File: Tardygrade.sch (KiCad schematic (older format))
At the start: 25 parts, among them J1 Conn_01x03, J2 Conn_01x03, J3 Conn_01x03, J4 Conn_01x03, Q1 FET, Q2 FET, U1 MCP1642B, U2 HUZZAH32, U3 Tinypico, U4 HallSwitch, U5 HallSwitch, U6 HallSwitch, U7 HallSwitch, X1 XpansionHeader

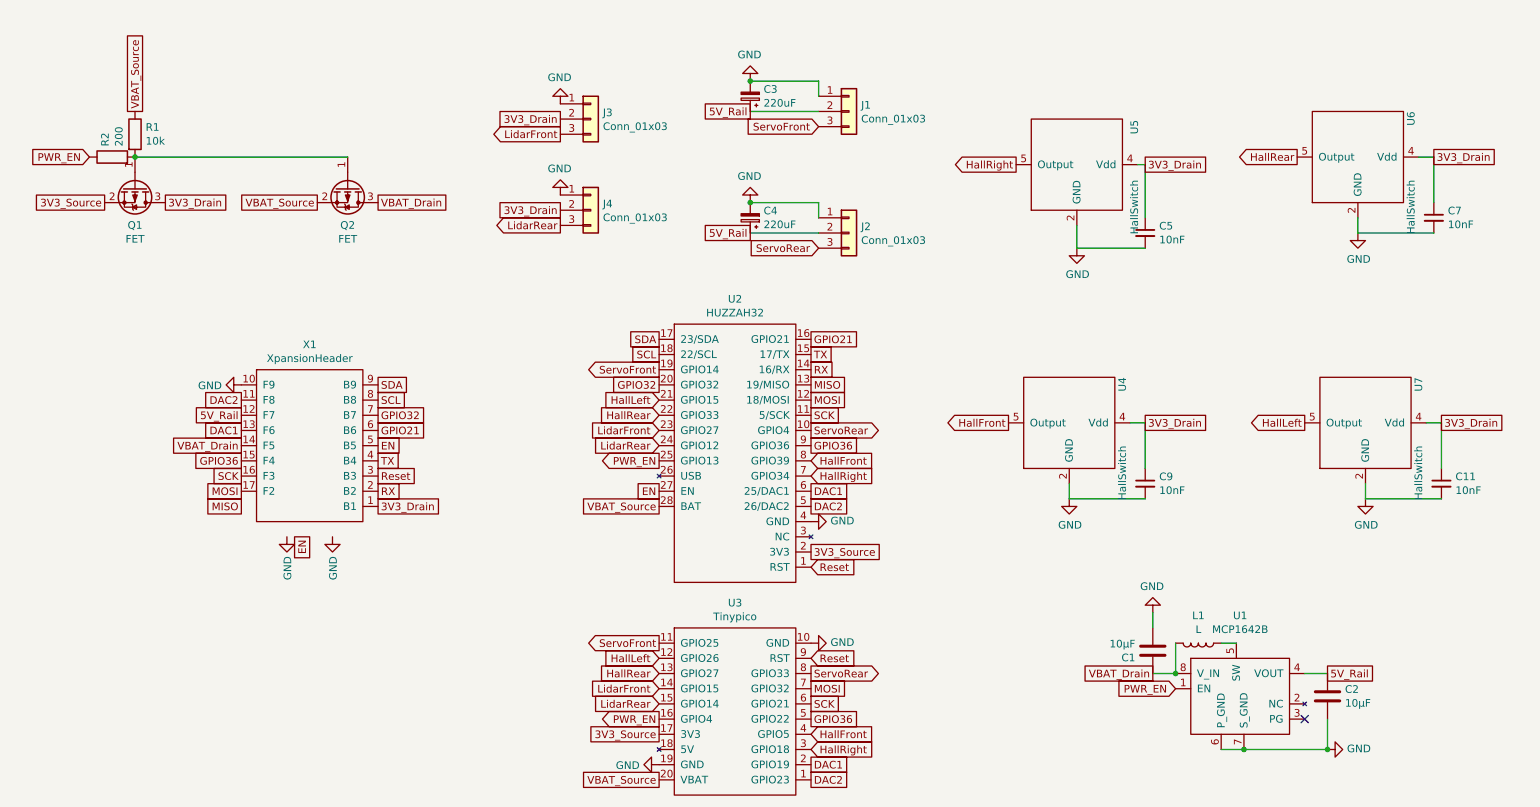
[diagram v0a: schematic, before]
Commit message: Changed some GPIOs. Minor edits.
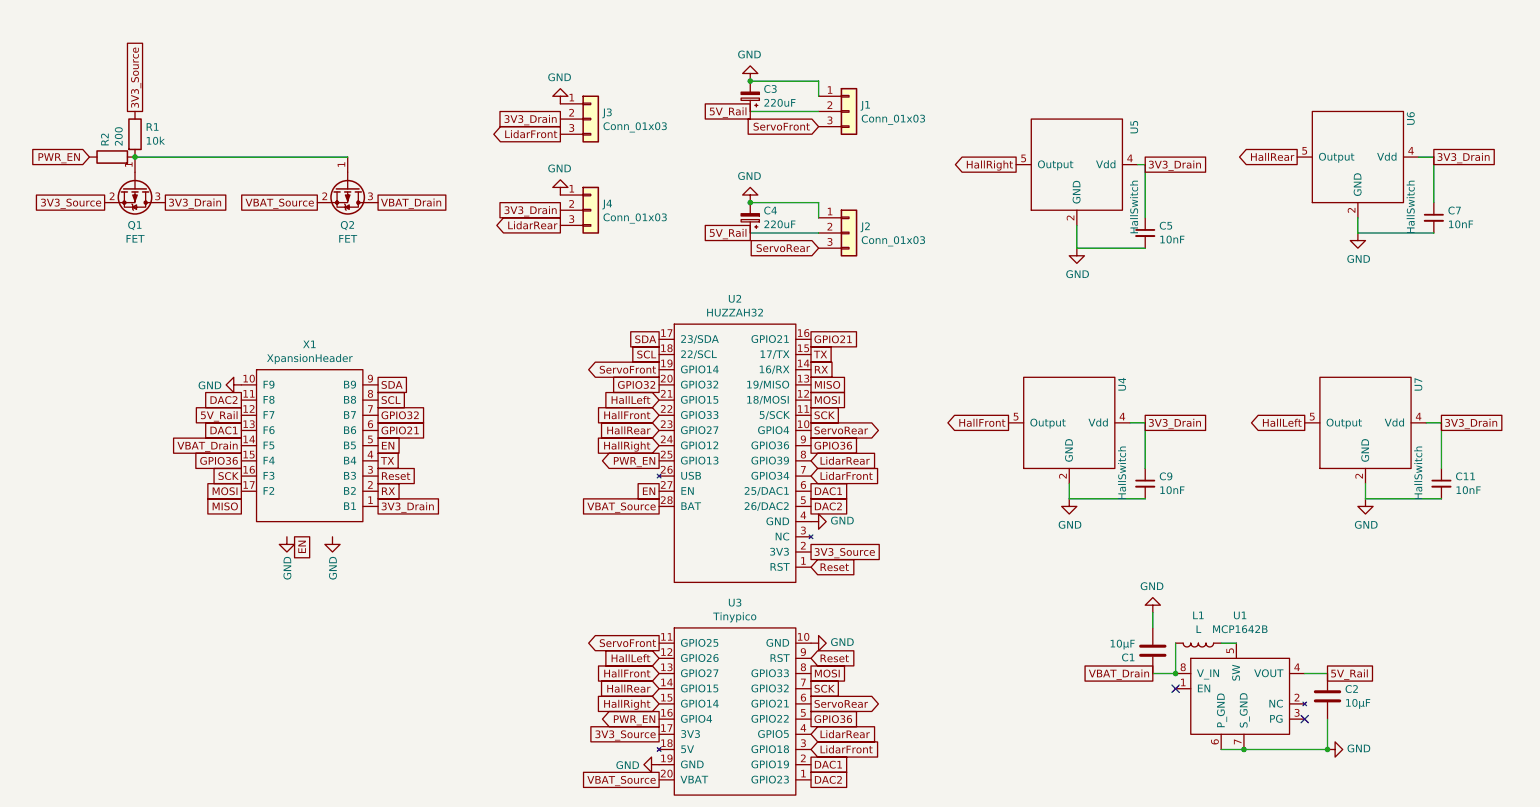
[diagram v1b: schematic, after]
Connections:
- net 3V3_Source: now also R1.1
- net HallFront: now also U2.22 (GPIO33), U3.13 (GPIO27); no longer U2.8 (GPIO39), U3.4 (GPIO5)
- net HallRear: now also U2.23 (GPIO27), U3.14 (GPIO15); no longer U2.22 (GPIO33), U3.13 (GPIO27)
- net HallRight: now also U2.24 (GPIO12), U3.15 (GPIO14); no longer U2.7 (GPIO34), U3.3 (GPIO18)
- net LidarFront: now also U2.7 (GPIO34), U3.3 (GPIO18); no longer U2.23 (GPIO27), U3.14 (GPIO15)
- net LidarRear: now also U2.8 (GPIO39), U3.4 (GPIO5); no longer U2.24 (GPIO12), U3.15 (GPIO14)
- net MOSI: now also U3.8 (GPIO33); no longer U3.7 (GPIO32)
- net PWR_EN: no longer U1.1 (EN)
- net SCK: now also U3.7 (GPIO32); no longer U3.6 (GPIO21)
- net ServoRear: now also U3.6 (GPIO21); no longer U3.8 (GPIO33)
- net VBAT_Source: no longer R1.1
- no-connect marks 1 -> 2
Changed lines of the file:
@@
 encoding utf-8
 Sheet 1 1
-Title ""
-Date ""
+Title "Tardygrade pcb v0.31"
+Date "2021-10-11"
 Rev ""
 Comp ""
@@
 Text GLabel 9750 3250 0    50   Output ~ 0
 HallLeft
-Text GLabel 5500 3200 0    50   Input ~ 0
+Text GLabel 5500 3300 0    50   Input ~ 0
 HallRear
 Text GLabel 9700 1500 0    50   Output ~ 0
 HallRear
-Text GLabel 6500 5300 2    50   Input ~ 0
+Text GLabel 5500 4900 0    50   Input ~ 0
 HallFront
-Text GLabel 6500 3500 2    50   Input ~ 0
+Text GLabel 5500 3200 0    50   Input ~ 0
 HallFront
 Text GLabel 7800 3250 0    50   Output ~ 0
 HallFront
-Text GLabel 6500 5400 2    50   Input ~ 0
+Text GLabel 5500 5100 0    50   Input ~ 0
 HallRight
-Text GLabel 6500 3600 2    50   Input ~ 0
+Text GLabel 5500 3400 0    50   Input ~ 0
 HallRight
 Text GLabel 7850 1550 0    50   Output ~ 0
@@
 Text GLabel 4850 1350 0    50   Output ~ 0
 LidarFront
-Text GLabel 5500 3300 0    50   Input ~ 0
+Text GLabel 6500 3600 2    50   Input ~ 0
 LidarFront
 $Comp
@@
 Text GLabel 1750 1500 0    50   Input ~ 0
 PWR_EN
-Text GLabel 8900 5000 0    50   Input ~ 0
-PWR_EN
 $Comp
 L power:GND #PWR0105
@@
 	0    -1   -1   0
 $EndComp
+Text GLabel 6500 5400 2    50   Input ~ 0
+LidarFront
+Text GLabel 6500 5100 2    50   Output ~ 0
+ServoRear
 Text GLabel 5500 5000 0    50   Input ~ 0
-LidarFront
-Text GLabel 6500 4900 2    50   Output ~ 0
-ServoRear
-Text GLabel 5500 4900 0    50   Input ~ 0
 HallRear
 $Comp
@@
 Text GLabel 4850 1950 0    50   Output ~ 0
 LidarRear
-Text GLabel 5500 5100 0    50   Input ~ 0
+Text GLabel 6500 5300 2    50   Input ~ 0
 LidarRear
-Text GLabel 5500 3400 0    50   Input ~ 0
+Text GLabel 6500 3500 2    50   Input ~ 0
 LidarRear
 Text GLabel 6500 3300 2    50   Output ~ 0
@@
 Text GLabel 1850 1800 0    50   UnSpc ~ 0
 3V3_Source
-Text GLabel 3250 1800 0    50   UnSpc ~ 0
-VBAT_Source
 Text GLabel 8750 4900 0    50   UnSpc ~ 0
 VBAT_Drain
@@
 Text GLabel 6500 4800 2    50   Input ~ 0
 Reset
-Text GLabel 2050 1200 1    50   UnSpc ~ 0
-VBAT_Source
 Text GLabel 3650 3400 2    50   UnSpc ~ 0
 EN
@@
 	1    0    0    -1
 $EndComp
+Text GLabel 6500 4900 2    50   UnSpc ~ 0
+MOSI
 Text GLabel 6500 5000 2    50   UnSpc ~ 0
-MOSI
-Text GLabel 6500 5100 2    50   UnSpc ~ 0
 SCK
 Text GLabel 6500 5200 2    50   UnSpc ~ 0
@@
 	6550 1800 6550 1900
 Connection ~ 6100 1800
+NoConn ~ 8900 5000
+Text GLabel 3250 1800 0    50   UnSpc ~ 0
+VBAT_Source
+Text GLabel 2050 1200 1    50   UnSpc ~ 0
+3V3_Source
 $EndSCHEMATC
